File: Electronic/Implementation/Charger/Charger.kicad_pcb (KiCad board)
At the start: 2 copper layers, 46 x 28 mm, 16 parts, among them J1 Jack-DC, J2 66200221022, Q1 Q_PMOS_GSD, U1 MCP73844T-820I

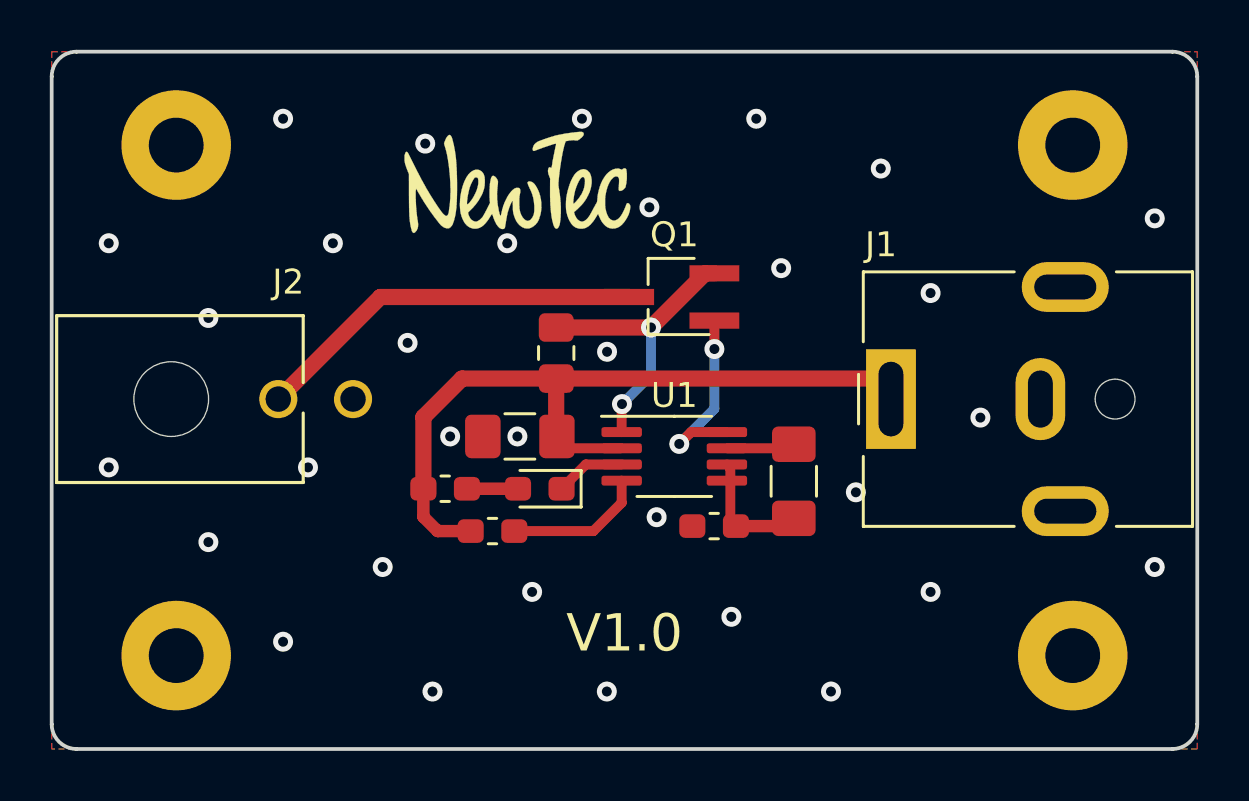
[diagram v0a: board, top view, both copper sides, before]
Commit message: Charger - save with KiCad 6.0
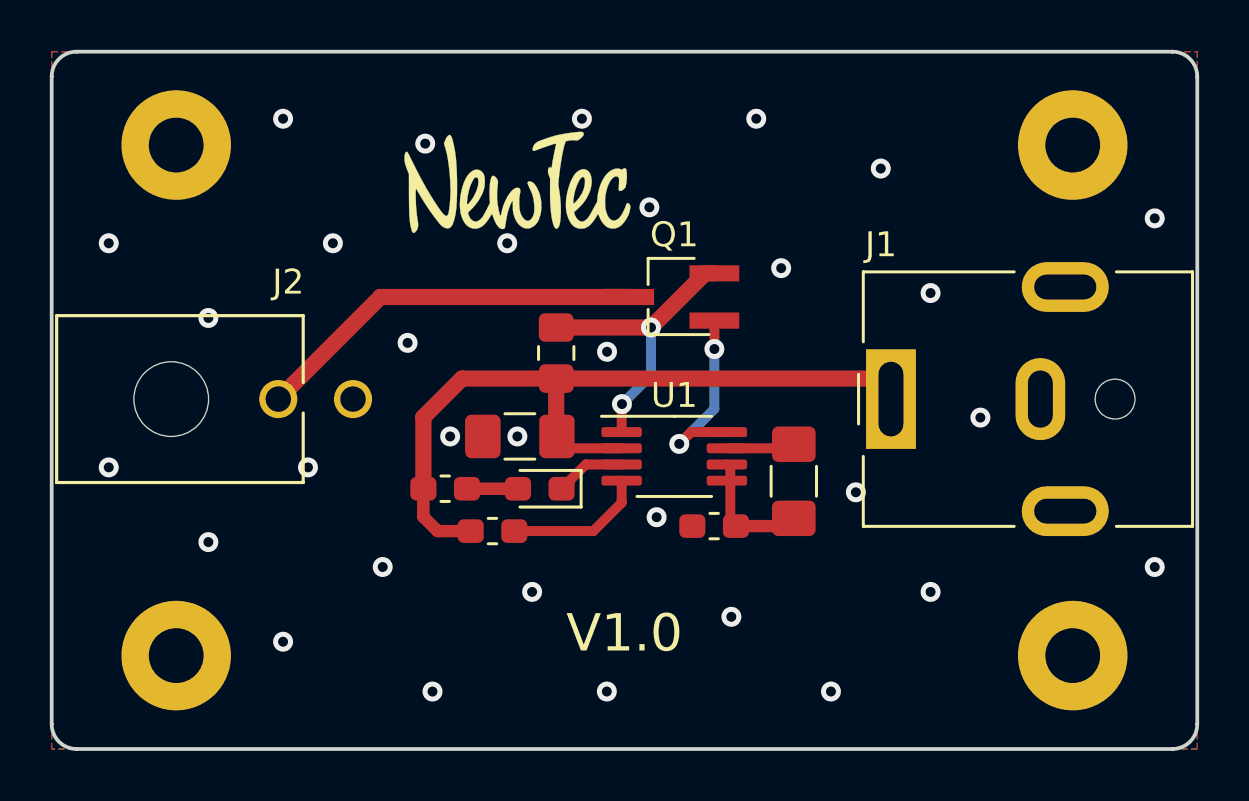
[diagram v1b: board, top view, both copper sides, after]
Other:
- net class Default removed
